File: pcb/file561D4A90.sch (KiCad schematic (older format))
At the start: 50 parts

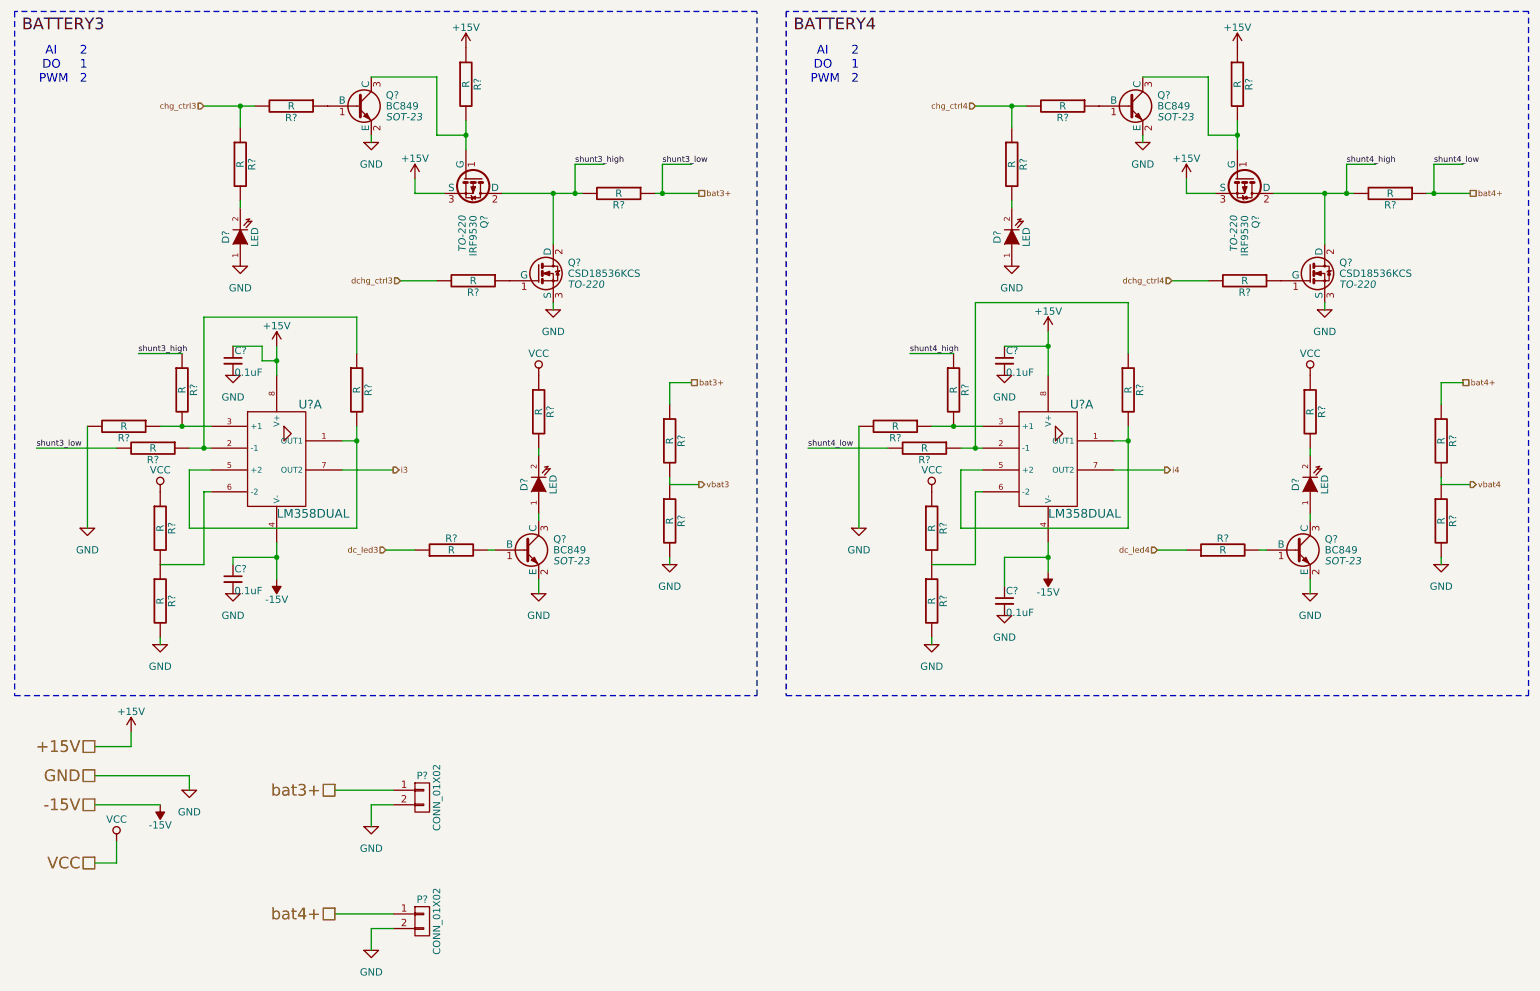
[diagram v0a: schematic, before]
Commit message: starting on layout
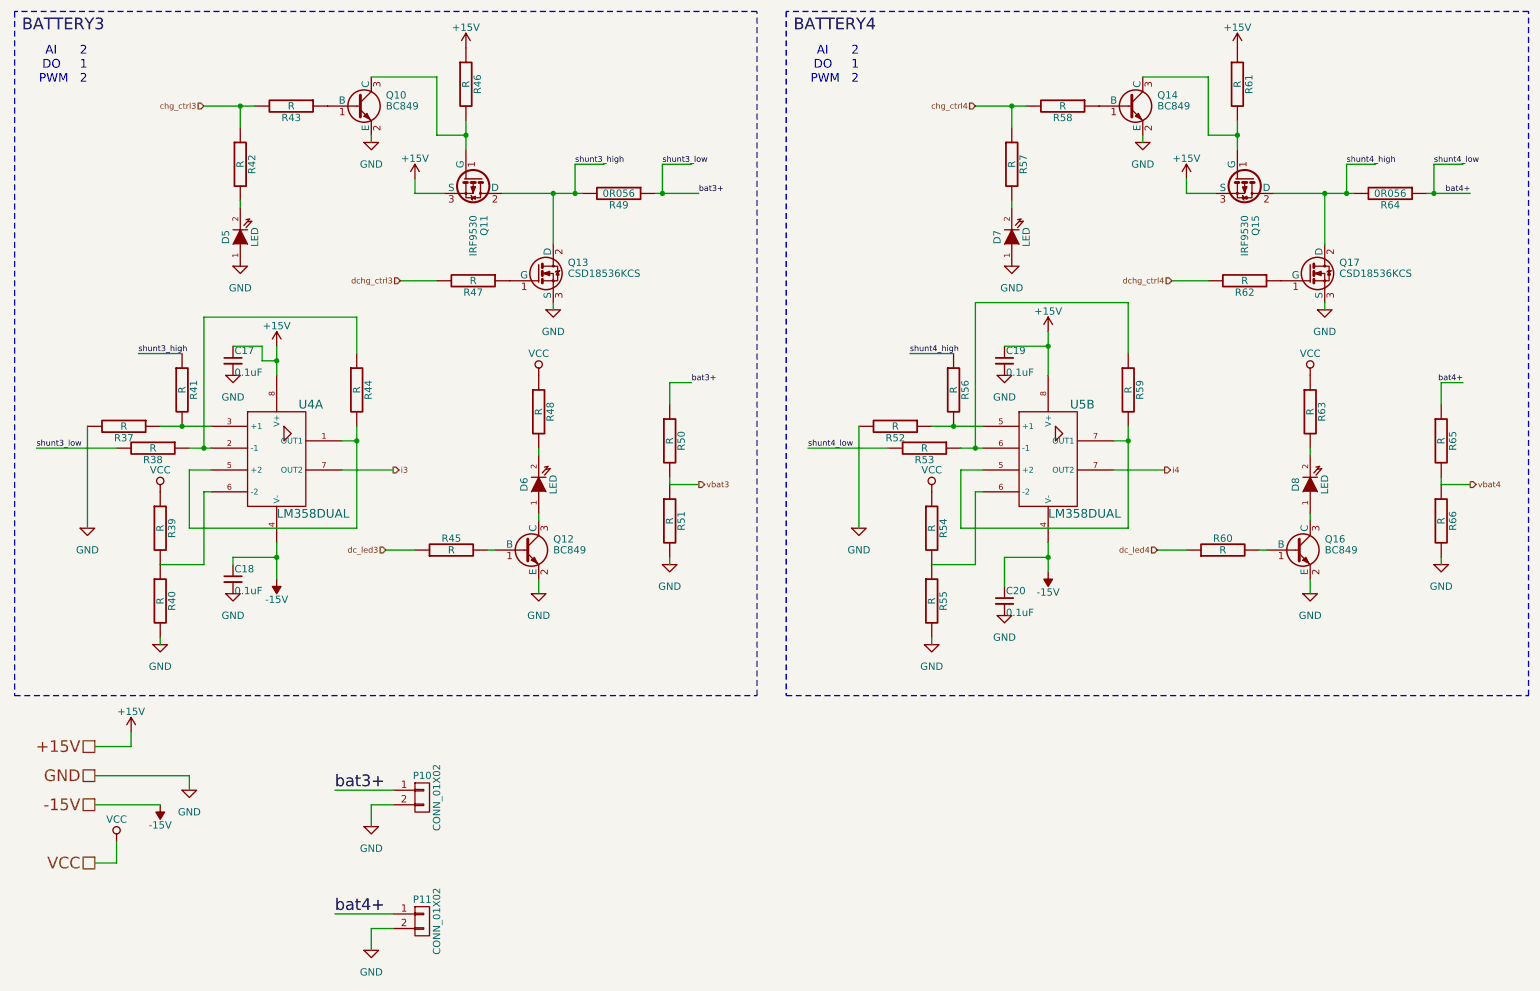
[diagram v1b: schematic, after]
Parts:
- C17, C18, C19, C20: renamed from C?; footprint (none) -> Capacitors_SMD:C_0805_HandSoldering
- D5, D6, D7, D8: renamed from D?; footprint (none) -> LEDs:LED-0805
- P10, P11: renamed from P?; footprint (none) -> Pin_Headers:Pin_Header_Straight_1x02
- Q10, Q12, Q14, Q16: renamed from Q?; footprint SOT-23 -> Housings_SOT-23_SOT-143_TSOT-6:SOT-23_Handsoldering
- Q11, Q13, Q15, Q17: renamed from Q?; footprint TO-220 -> Power_Integrations:TO-220
- R37, R38, R39, R40, R41, R44, R50, R51, R52, R53, R54, R55, R56, R59, R65, R66: renamed from R?; footprint (none) -> Resistors_ThroughHole:Resistor_Horizontal_RM10mm
- R42, R43, R45, R46, R47, R48, R57, R58, R60, R62, R63: renamed from R?; footprint (none) -> Resistors_SMD:R_0805_HandSoldering
- R49, R64: renamed from R?; value R -> 0R056; footprint (none) -> Resistors_SMD:R_2512_HandSoldering; Part # (none) -> RL2512 FK-07 0R056
- R61: renamed from R?; footprint (none) -> Resistors_SMD:R_2512_HandSoldering
- U4, U5: renamed from U?; footprint (none) -> Housings_SOIC:SOIC-8_3.9x4.9mm_Pitch1.27mm
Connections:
- net at R53.1, R59.1: now also U5.6 (-2); no longer U5.2 (-1)
- net at R52.1, R56.2: now also U5.5 (+2); no longer U5.3 (+1)
- new net: R59.2, U5.5 (+2), U5.7 (OUT2)
